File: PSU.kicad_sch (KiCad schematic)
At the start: 69 parts, among them J6 Conn_01x01_Socket, Q401 2N7002, SW401 SW_Push, SW402 SW_Push, U3 TPPM0110DWPR, U4 TPS548A23VANR, U402 AP7381-33SA-7, U403 AP63200WU

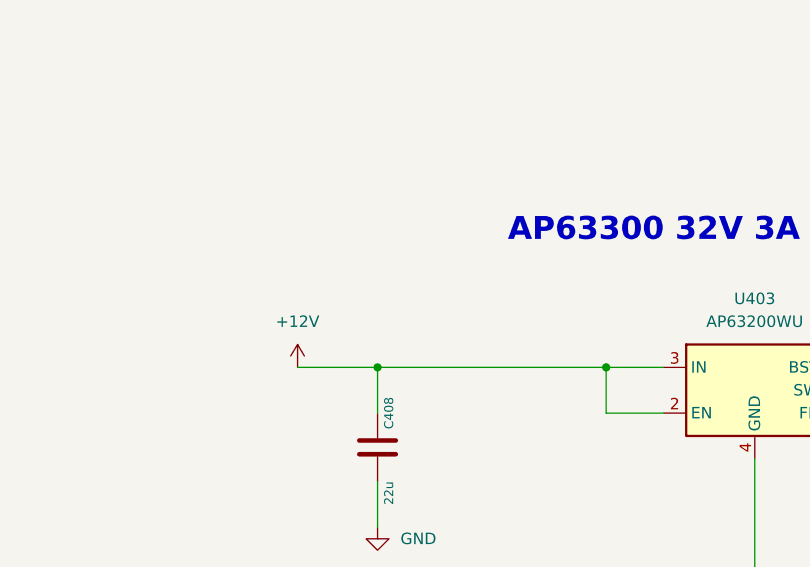
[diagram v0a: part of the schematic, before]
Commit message: Prototype
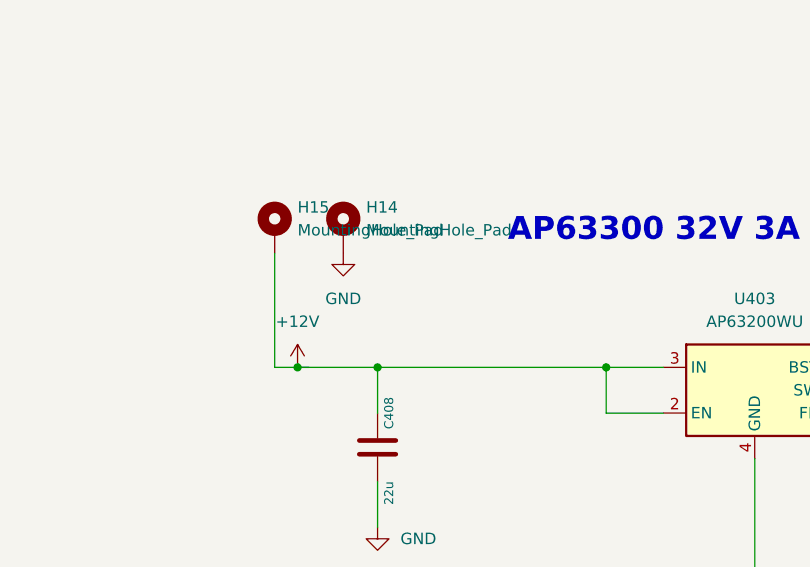
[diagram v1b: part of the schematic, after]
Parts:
- added H14, H15: MountingHole_Pad, Connector:Banana_Jack_1Pin, symbol Mechanical:MountingHole_Pad
- C416, C417: footprint A_HDJ_Library:C_0402_1005Metric -> A_DFRobot:C_0603; MPN GRM155R61H105KE05D -> GZ1608D601TF
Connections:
- net +12V: now also H15.1
- net GND: now also H14.1
